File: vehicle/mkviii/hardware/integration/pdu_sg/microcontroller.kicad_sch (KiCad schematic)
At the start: 15 parts, among them J1 J_Programming_Pin_Header, U1 STM32G441KBT6, U2 MCP2561-E_SN, Y1 X_16MHz_18pF

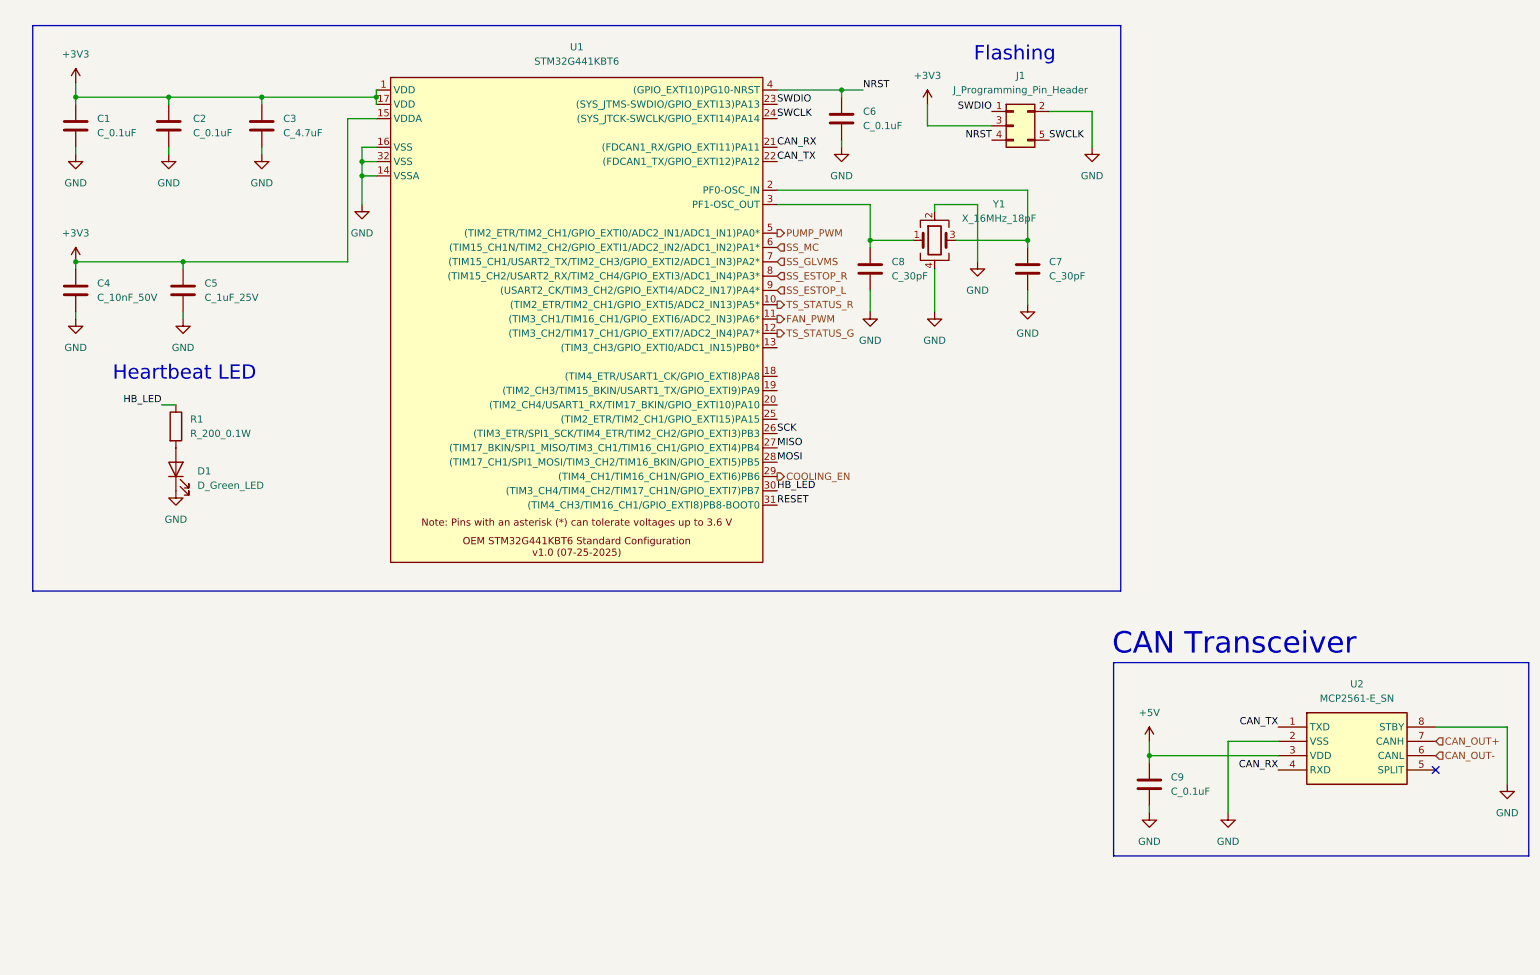
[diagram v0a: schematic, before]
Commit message: adc
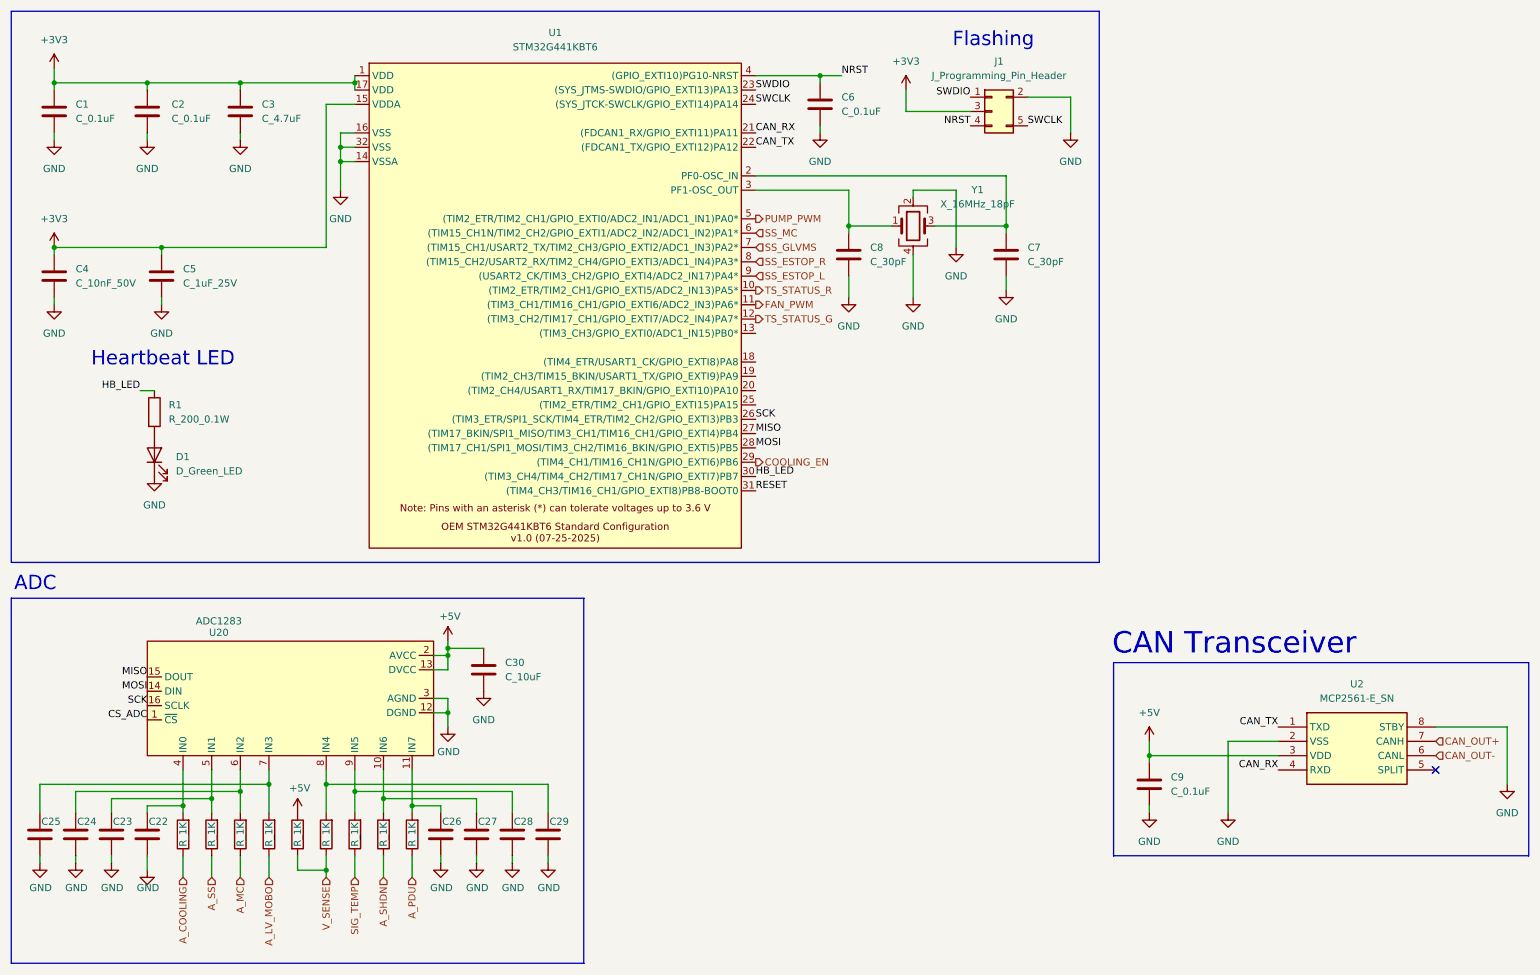
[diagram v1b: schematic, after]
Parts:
- added C22, C23, C24, C25, C26, C27, C28, C29: C_10uF, OEM:C_0603, symbol OEM:C_10uF
- added C30: C_10uF, OEM:C_0603_1608Metric, symbol OEM:C_10uF_10V_0603
- added R18, R20, R45, R54, R55, R56, R57, R58, R59: R_1K, OEM:R_0603, symbol OEM:R_1K
- added U20: ADC1283, Package_SO:TSSOP-16_4.4x5mm_P0.65mm, symbol Analog_ADC:ADC1283
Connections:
- net +5V: now also C30.1, R45.1, U20.13 (DVCC), U20.2 (AVCC)
- net GND: now also C22.2, C23.2, C24.2, C25.2, C26.2, C27.2, C28.2, C29.2, C30.2, U20.12 (DGND), U20.3 (AGND)
- net MISO: now also U20.15 (DOUT)
- net MOSI: now also U20.14 (DIN)
- net SCK: now also U20.16 (SCLK)
- new net: C25.1, R55.2, U20.7 (IN3)
- new net: C24.1, R54.2, U20.6 (IN2)
- new net: C27.1, R58.2, U20.10 (IN6)
- new net: C26.1, R59.2, U20.11 (IN7)
- new net: C22.1, R18.2, U20.4 (IN0)
- new net: C23.1, R20.2, U20.5 (IN1)
- new net: C29.1, R56.2, U20.8 (IN4)
- new net: C28.1, R57.2, U20.9 (IN5)
- new net A_COOLING: R18.1
- new net A_LV_MOBO: R55.1
- new net A_MC: R54.1
- new net A_PDU: R59.1
- new net A_SHDN: R58.1
- new net A_SS: R20.1
- new net CS_ADC: U20.1 (~{CS})
- new net SIG_TEMP: R57.1
- new net V_SENSE: R45.2, R56.1
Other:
- note added: "ADC"
- moved on the sheet: C1, C2, C3, C4, C5, C6, C7, C8, D1, J1, R1, U1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
